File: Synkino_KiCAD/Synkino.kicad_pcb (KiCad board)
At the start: 2 copper layers, 93.3 x 82.3 mm, 186 parts, among them J1 Pwr, J10 EYE8_OUT, J11 EYE4_OUT, J12 2.5mm, J13 EYE5_OUT, J2 2.5mm, J3 3.5mm, J4 Micro_SD_Card_Det_Hirose_DM3AT, J5 EYE1_OUT, J6 EYE6_OUT, J7 EYE2_OUT, J8 EYE7_OUT, J9 EYE3_OUT, Q1 IRF7319, Q2 BC847, Q3 IRLML2244, SW1 SW_Push, SW2 Rotary_Encoder_Switch, SW3 SW_Push, U1 MCP1702T-5002E/MB, U10 ATMEGA328P-AU, U11 QRE1113, U12 QRE1113, U13 QRE1113, U14 QRE1113, U15 QRE1113, U16 QRE1113, U17 24LC256, U18 QRE1113, U2 ATMEGA328P-AU, U3 74HC4050, U4 SPIOLED128x64, U5 AP7312-1833W6-7, U6 74HC14, U7 VS1053B, U8 MAX4741, U9 QRE1113, X1 FTDIconn, X2 ICSP, X3 FTDIconn, X4 ICSP, Y1 16Mhz, Y2 12.288MHz, Y3 16Mhz

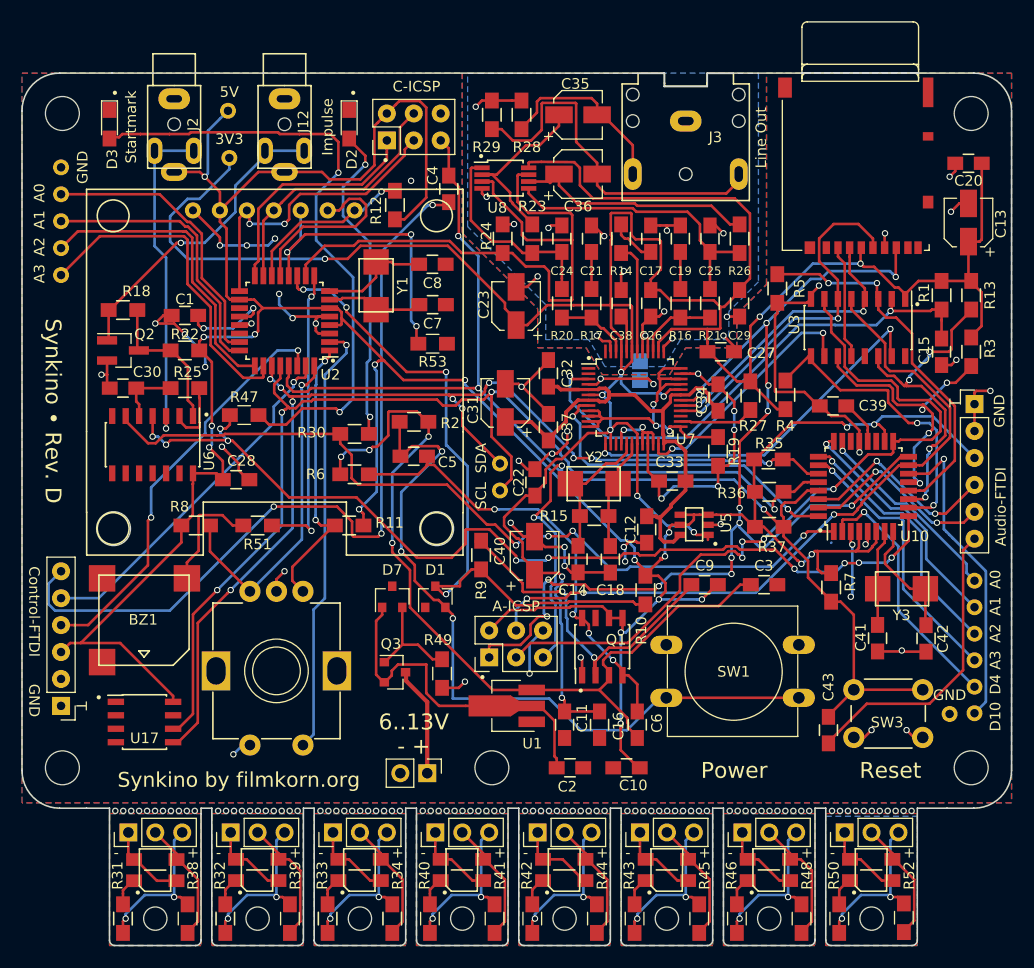
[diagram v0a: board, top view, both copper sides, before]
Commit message: KiCad 5 version, .gitignore
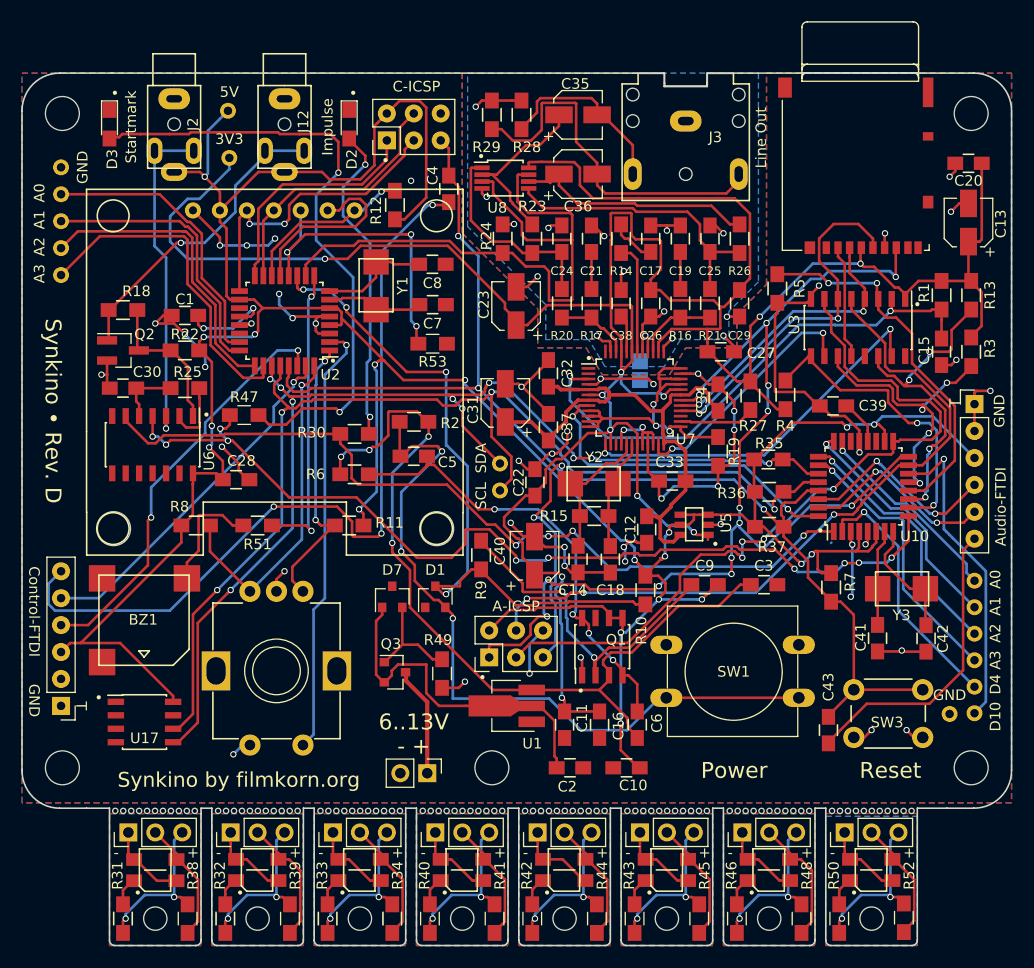
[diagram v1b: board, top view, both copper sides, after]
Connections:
- net /~PWR_OFF renamed /~{PWR_OFF}
- net /~RST renamed /~{RST}
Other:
- net class Default removed
